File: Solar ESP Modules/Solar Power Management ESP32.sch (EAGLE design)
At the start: 54 parts, among them IC1 TP4056, IC2 1117-33, IC5 1117-33, J3 USB-C-Socket, Q1 FDN360P, T3 MBT2N2222, T4 MBT2N2222, U2 ESP-WROOM-32NARROW, U6 FT232RLSSOP

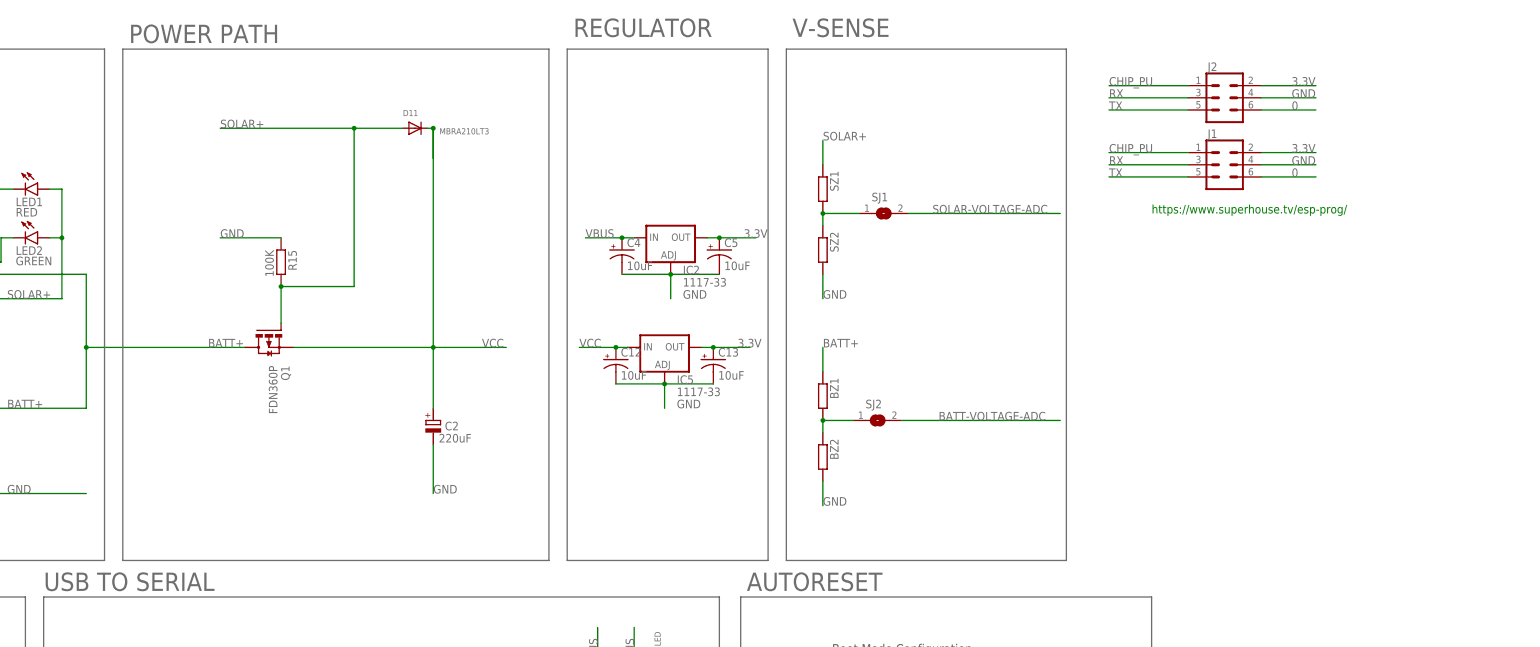
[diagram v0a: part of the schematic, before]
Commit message: update
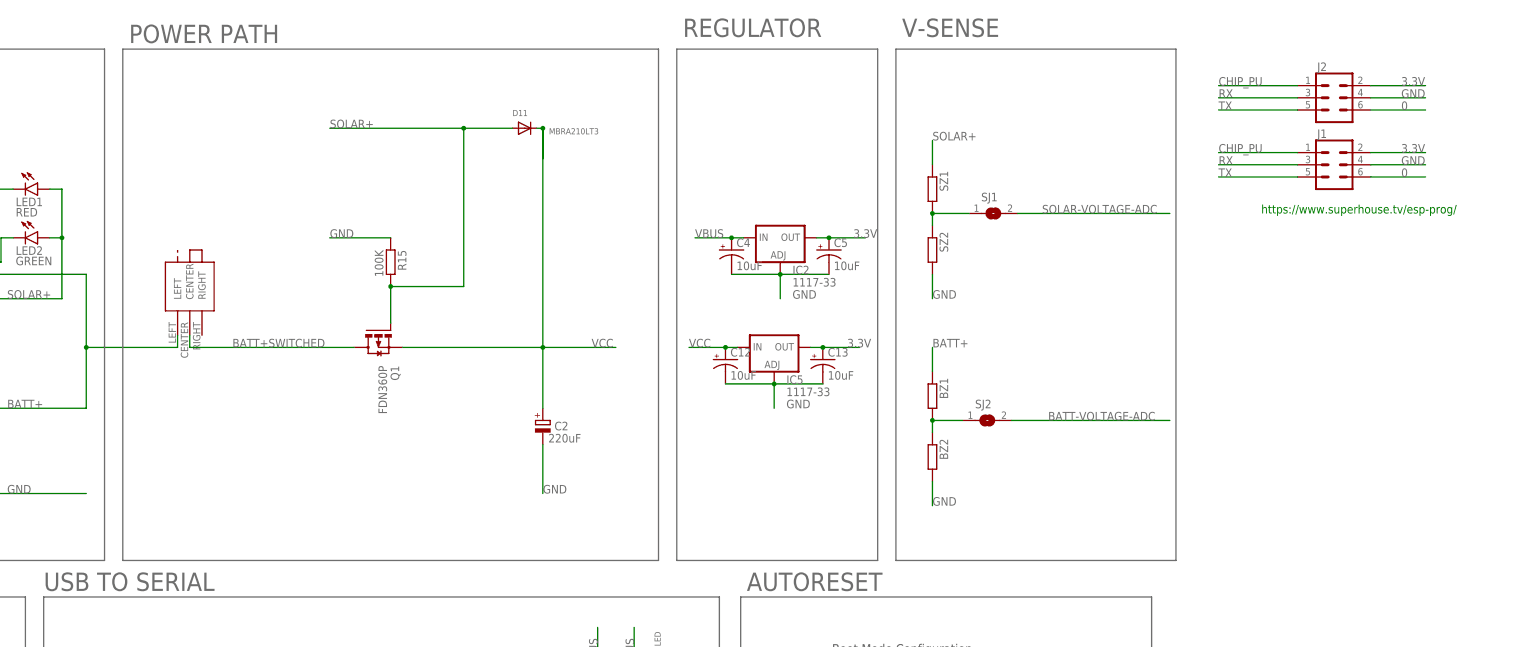
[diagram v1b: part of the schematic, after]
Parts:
- added U$3: XKBENTERPRISESS-12D11G5R, XKB Enterprise SS-12D11G5R:XKBENTERPRISESS-12D11G5R
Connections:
- new net BATT+SWITCHED: Q1.D, U$3.CENTER
- net BATT+: now also U$3.LEFT; no longer Q1.D
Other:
- moved on the sheet: BZ1, BZ2, C12, C13, C2, C4, C5, D11, IC2, IC5, J1, J2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
